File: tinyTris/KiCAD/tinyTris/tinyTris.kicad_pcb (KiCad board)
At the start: 2 copper layers, 64.1 x 42.5 mm, 15 parts, among them SW1 Reset, SW2 Rotate, SW3 Left, SW4 Right, SW5 Drop, U1 ATtiny85-20P, U2 SSD1306_I2C_display, U3 SSD1306_I2C_display

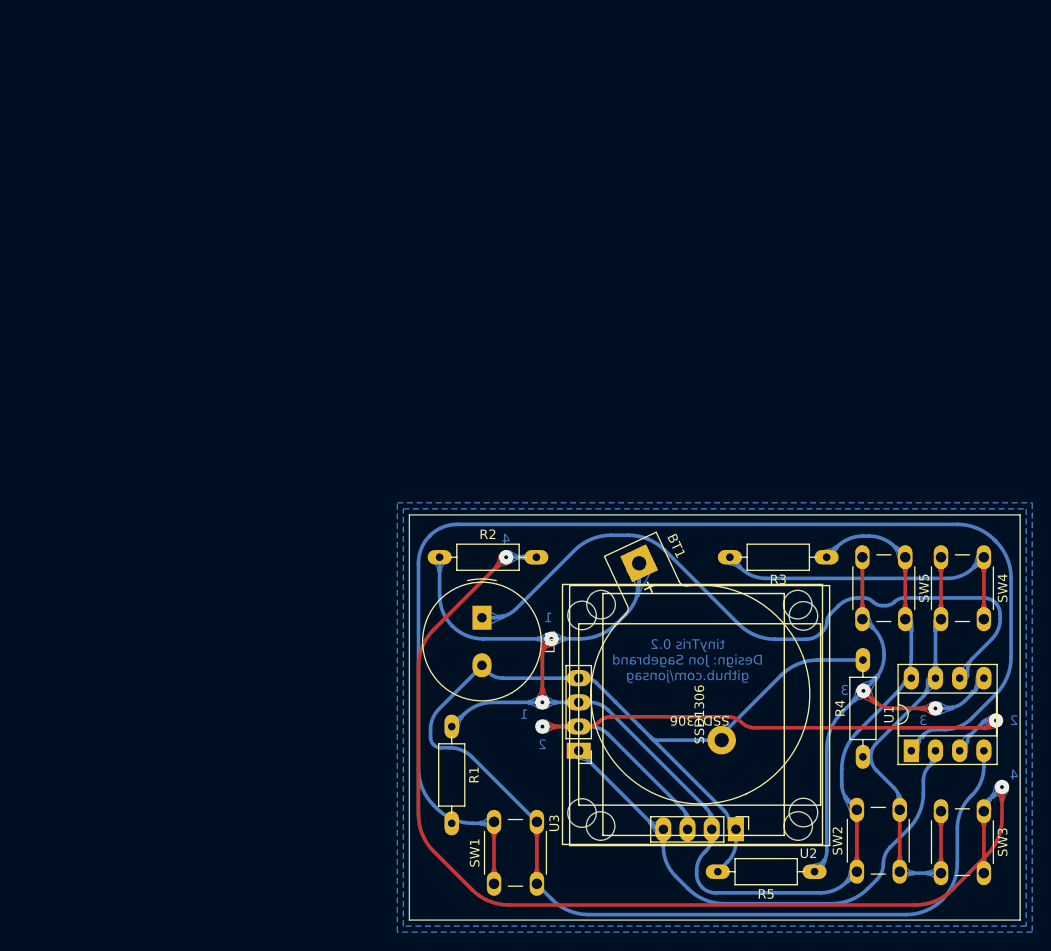
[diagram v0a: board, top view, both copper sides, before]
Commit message: new schematics
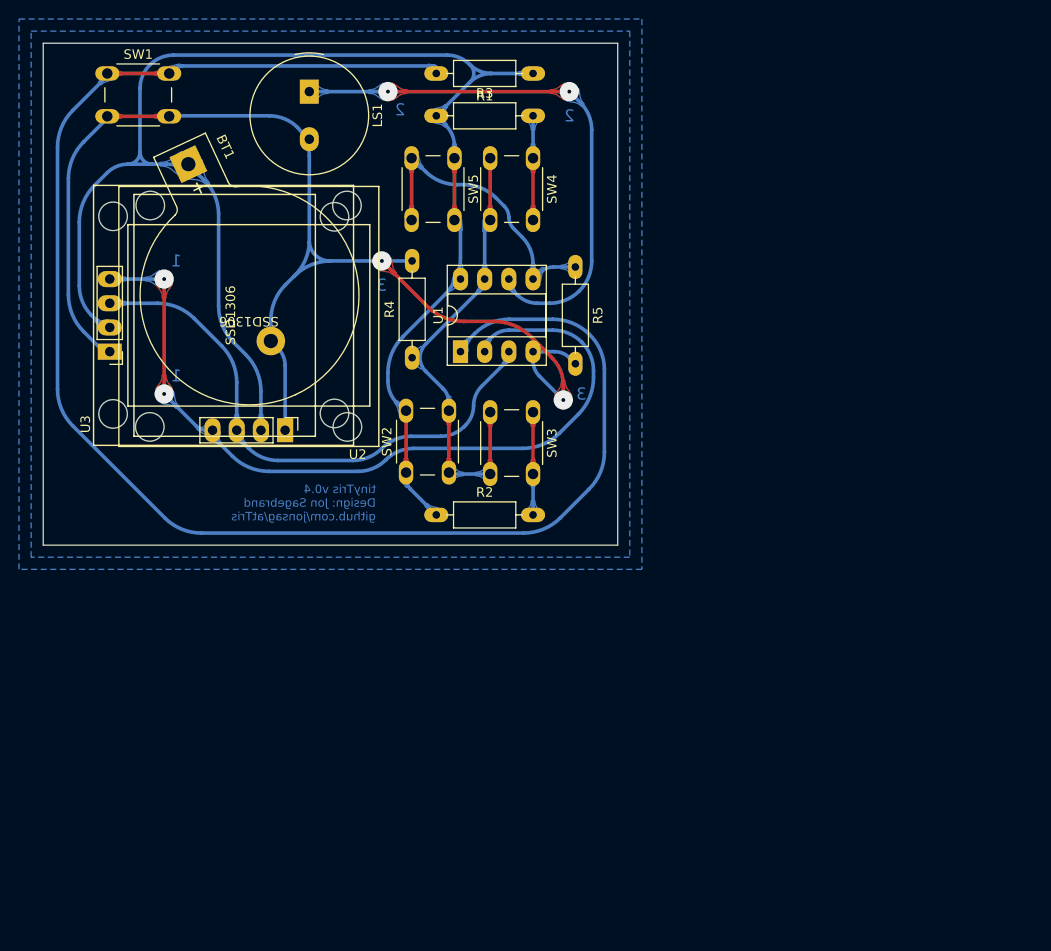
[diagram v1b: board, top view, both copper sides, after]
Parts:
- moved SW1 94.3 mm to (77.5, 71.1), turned to 0 degrees
- moved R1 69.1 mm to (122.2, 71.1), turned to 180 degrees
- moved R5 68.3 mm to (126.7, 91.4), turned to -90 degrees
- moved U3 64.7 mm to (77.8, 100.3)
- moved U1 63.2 mm to (114.6, 100.3)
- moved SW2 63.2 mm to (108.9, 113.0)
- moved BT1 63.2 mm to (86.0, 80.6)
- moved R4 63.2 mm to (109.5, 101.0)
- moved SW3 63.2 mm to (122.2, 106.7)
- moved SW4 63.2 mm to (122.2, 80.0)
- moved SW5 63.2 mm to (114.0, 80.0)
- moved U2 63.2 mm to (96.2, 108.6)
- moved R3 61.9 mm to (112.0, 75.6), turned to 0 degrees
- moved LS1 58.1 mm to (98.7, 73.0)
- moved R2 4.46 mm to (112.0, 117.5)
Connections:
- U3 pad 1: Net-(U1-Pad2) -> GND
- U3 pad 2: Net-(U1-Pad3) -> Net-(BT1-Pad1)
- U3 pad 3: Net-(BT1-Pad1) -> Net-(U1-Pad3)
- U3 pad 4: GND -> Net-(U1-Pad2)
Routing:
- net Net-(R2-Pad2): track 117.4 -> 10.8 mm, vias 2 -> 0
- net Net-(R1-Pad2): track 130.5 -> 167.6 mm
- net Net-(U1-Pad2): track 55.7 -> 86.3 mm, vias 0 -> 2
- net Net-(R3-Pad2): track 34.6 -> 10.8 mm
- net Net-(BT1-Pad1): track 144.5 -> 168.2 mm, vias 2 -> 0
- net Net-(R5-Pad1): track 51.7 -> 30.3 mm, vias 2 -> 0
- net GND: track 156.4 -> 135.7 mm, vias 0 -> 2
- net Net-(U1-Pad3): track 74.2 -> 57.7 mm, vias 2 -> 0
- net Net-(LS1-Pad1): track 73.6 -> 58.4 mm, vias 0 -> 2
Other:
- board size 64.1 x 42.5 mm -> 60.3 x 52.7 mm
- board text added: "tinyTris v0.4 Design: Jon Sagebrand github.com/jonsag/atTris"
- board text removed: "4"
- board text removed: "tinyTris 0.2 Design: Jon Sagebrand github.com/jonsag"
